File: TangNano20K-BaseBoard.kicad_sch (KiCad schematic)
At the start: 48 parts, among them J1 Conn_01x20_Socket, J2 Conn_01x20_Socket, J3 Conn_02x06_Odd_Even, Q1 PN2222A, Q2 PN2222A, Q3 PN2222A, Q4 PN2222A, SW1 SW_SPDT_321, SW2 SW_SPDT_321, SW3 SW_SPDT_321, SW4 SW_SPDT_321, SW5 SW_SPDT_321, U1 CC56-12EWA, U2 SSD1306

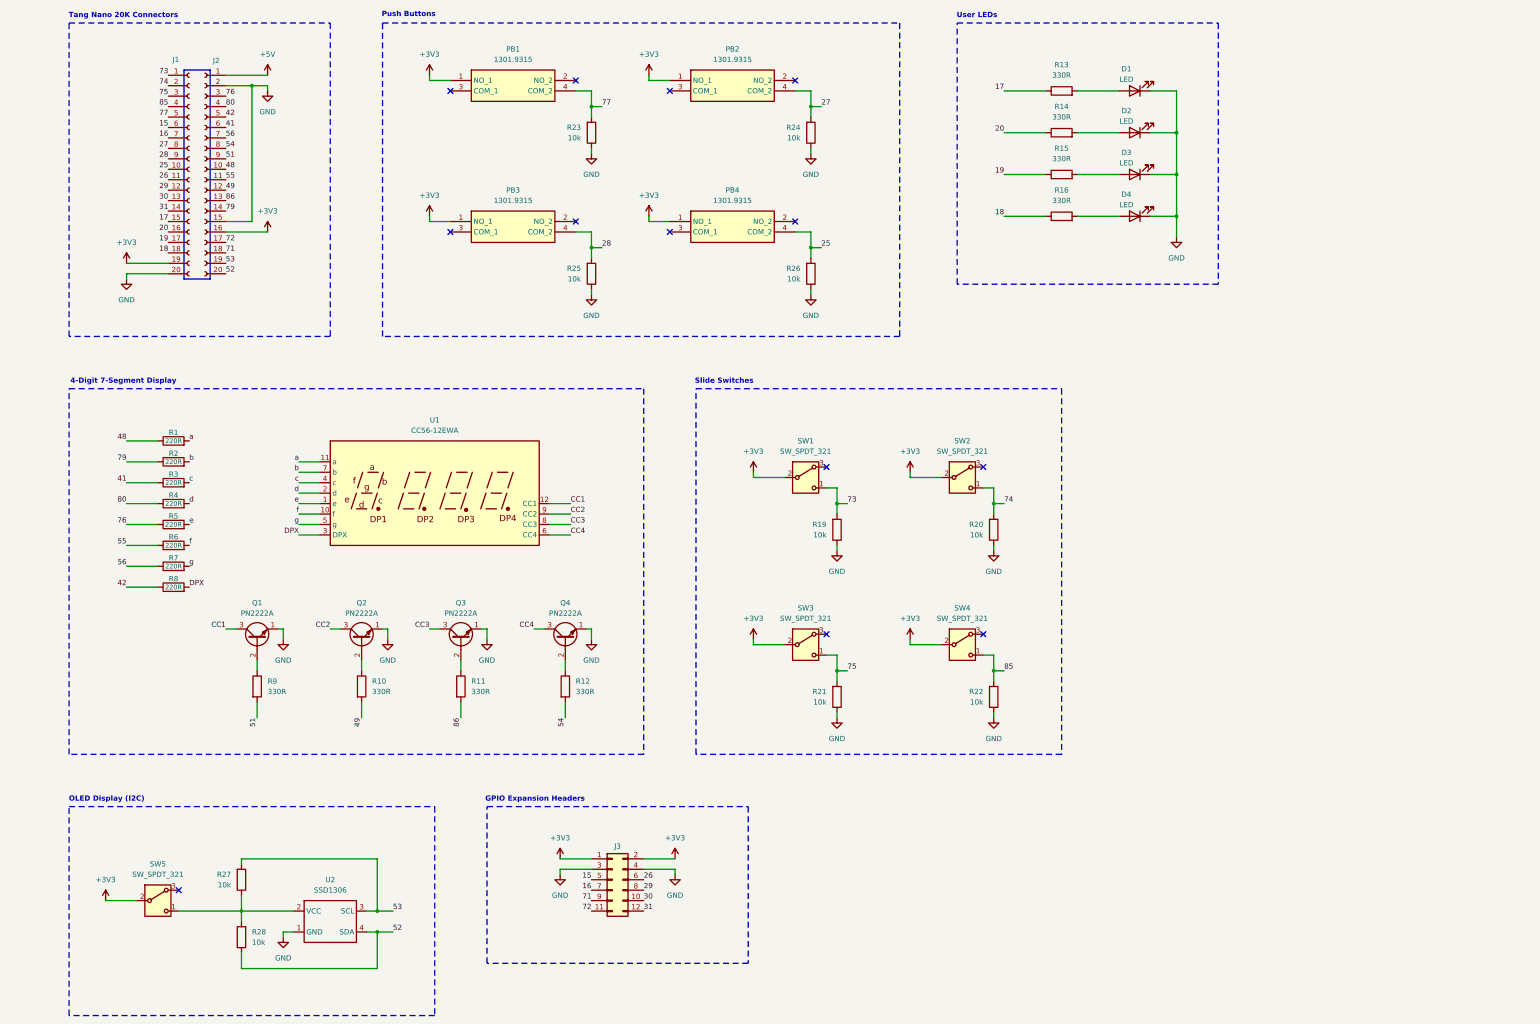
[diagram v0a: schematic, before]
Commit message: Update schematic
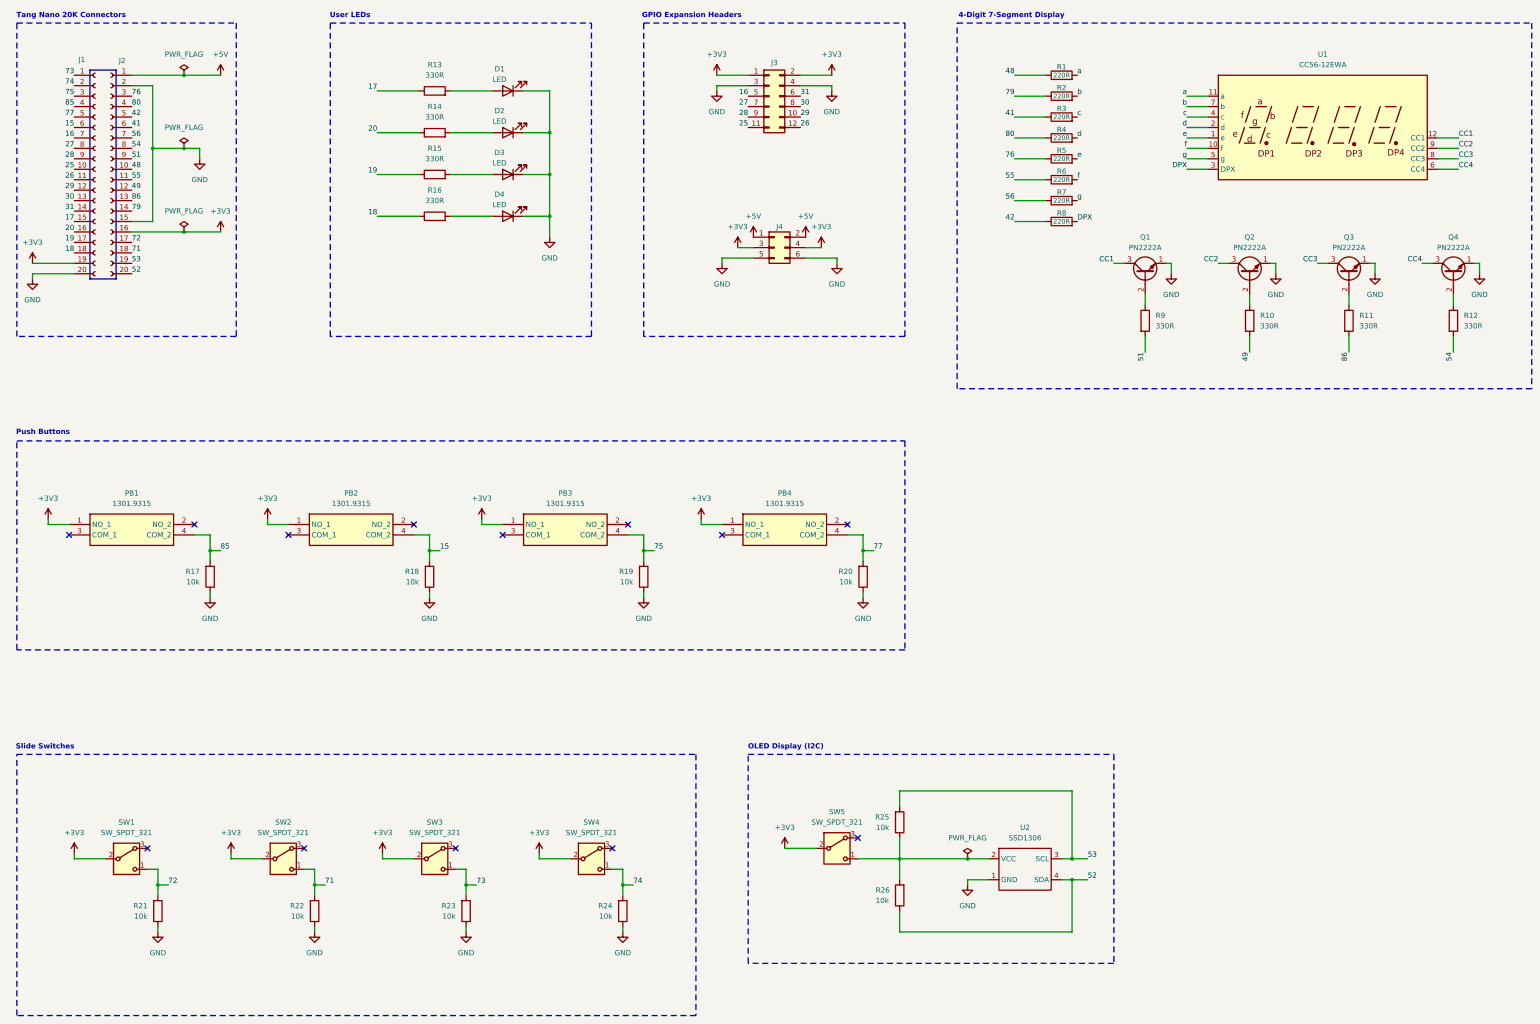
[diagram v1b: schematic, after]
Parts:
- added J4: Conn_02x03_Odd, Connector_PinSocket_2.54mm:PinSocket_2x03_P2.54mm_Horizontal, symbol Connector_Generic:Conn_02x03_Odd_Even
- renumbered R23 to R17, R24 to R18, R25 to R19, R26 to R20, R19 to R21, R20 to R22, R21 to R23, R22 to R24, R27 to R25, R28 to R26
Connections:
- net +3V3: now also J4.3 (Pin_3), J4.4 (Pin_4)
- net +5V: now also J4.1 (Pin_1), J4.2 (Pin_2)
- net 15: now also PB2.4 (COM_2), R18.2; no longer J3.5 (Pin_5)
- net 16: now also J3.5 (Pin_5); no longer J3.7 (Pin_7)
- net 25: now also J3.11 (Pin_11); no longer PB4.4 (COM_2), R20.2
- net 26: now also J3.12 (Pin_12); no longer J3.6 (Pin_6)
- net 27: now also J3.7 (Pin_7); no longer PB2.4 (COM_2), R18.2
- net 28: now also J3.9 (Pin_9); no longer PB3.4 (COM_2), R19.2
- net 29: now also J3.10 (Pin_10); no longer J3.8 (Pin_8)
- net 30: now also J3.8 (Pin_8); no longer J3.10 (Pin_10)
- net 31: now also J3.6 (Pin_6); no longer J3.12 (Pin_12)
- net 71: now also R22.2, SW2.1 (C); no longer J3.9 (Pin_9)
- net 72: now also R21.2, SW1.1 (C); no longer J3.11 (Pin_11)
- net 73: now also R23.2, SW3.1 (C); no longer R21.2, SW1.1 (C)
- net 74: now also R24.2, SW4.1 (C); no longer R22.2, SW2.1 (C)
- net 75: now also PB3.4 (COM_2), R19.2; no longer R23.2, SW3.1 (C)
- net 77: now also PB4.4 (COM_2), R20.2; no longer PB1.4 (COM_2), R17.2
- net 85: now also PB1.4 (COM_2), R17.2; no longer R24.2, SW4.1 (C)
- net GND: now also J4.5 (Pin_5), J4.6 (Pin_6)
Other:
- company: (none) -> Michał Głuszak
- title: (none) -> TangNano20K-BaseBoard
- moved on the sheet: D1, D2, D3, D4, J1, J2, J3, PB1, PB2, PB3, PB4, Q1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
